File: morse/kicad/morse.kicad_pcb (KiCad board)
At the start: 2 copper layers, 63.5 x 63.5 mm, 14 parts, among them J1 Conn_01x04, Q1 2N2219, Q2 2N2219

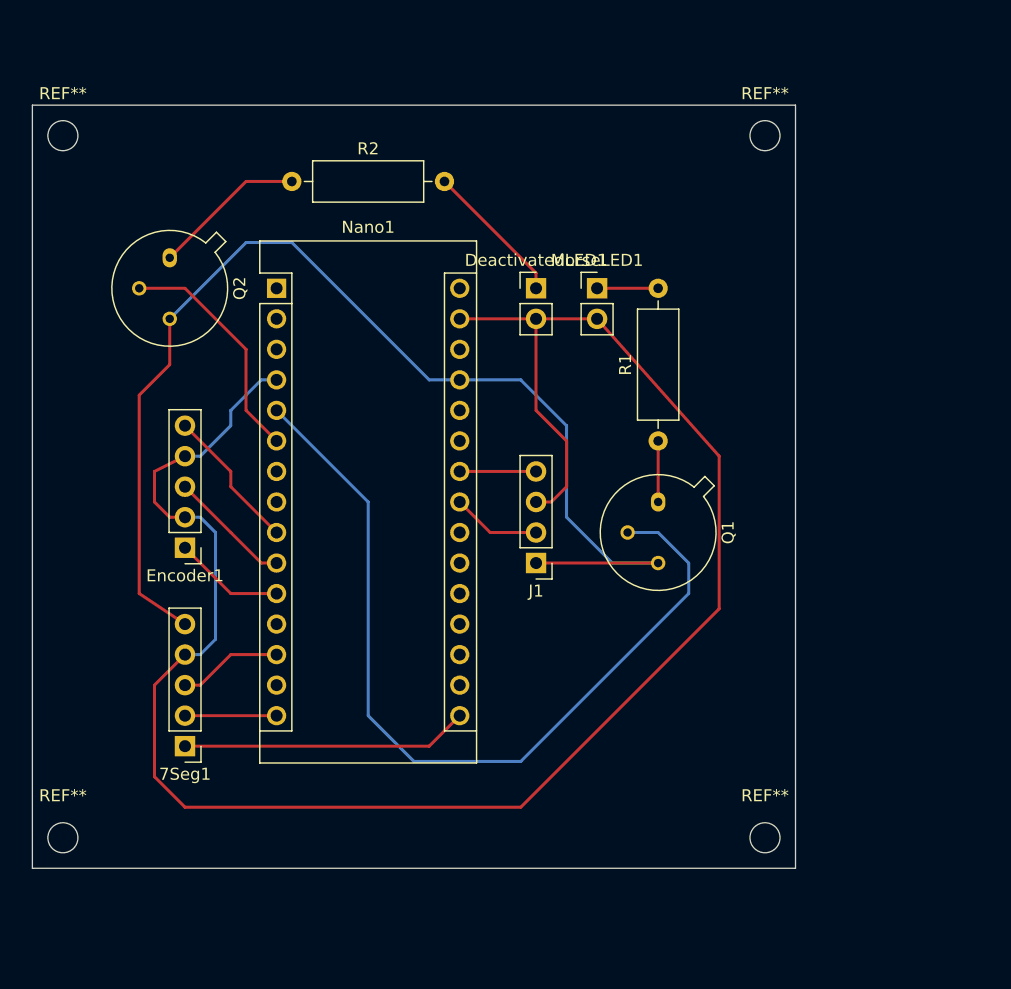
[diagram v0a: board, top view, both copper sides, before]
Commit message: updating morse pcb layout
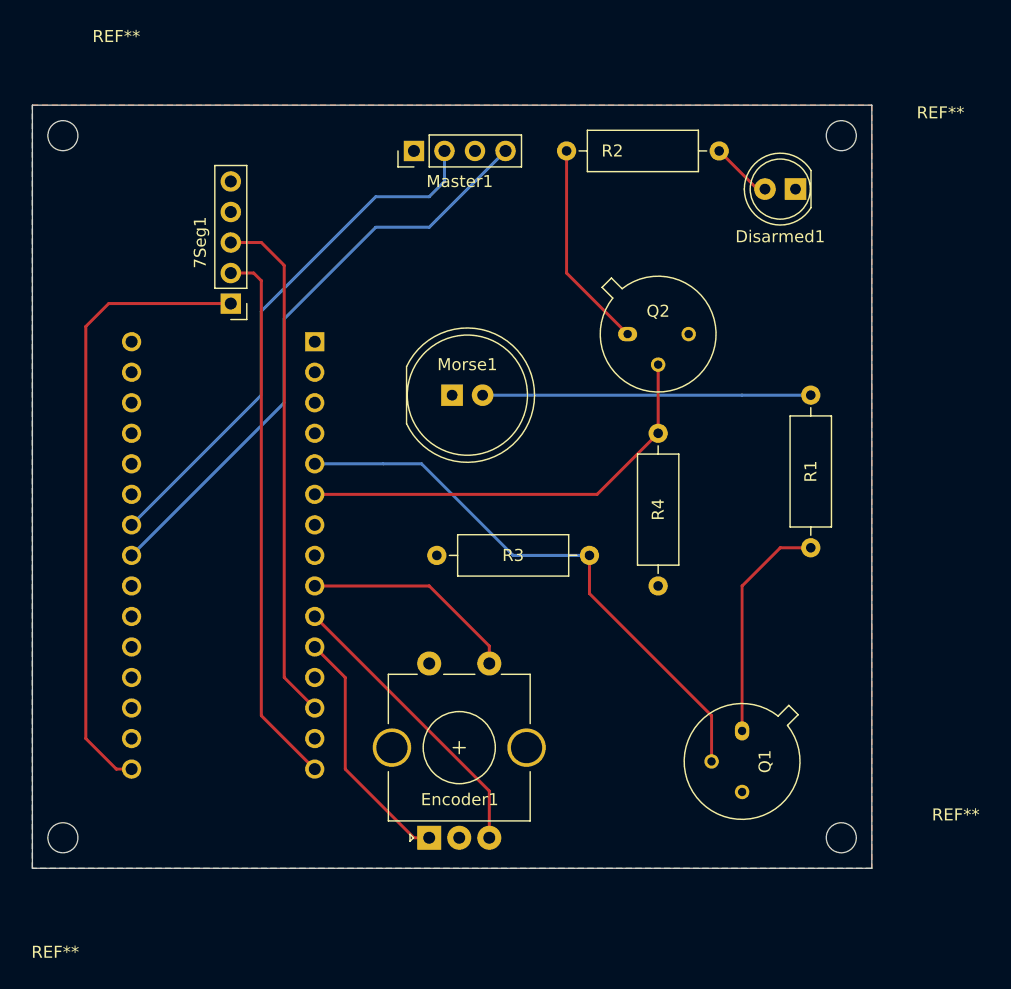
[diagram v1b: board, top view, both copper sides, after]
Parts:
- removed DeactivatedLED1, MorseLED1: Conn_01x02, Connector_PinHeader_2.54mm:PinHeader_1x02_P2.54mm_Vertical
- added Disarmed1: LED, LED_THT:LED_D5.0mm, F.Cu at (196.8, 78.1)
- added Morse1: LED, LED_THT:LED_D10.0mm, F.Cu at (168.3, 95.2)
- added R3: R, Resistor_THT:R_Axial_DIN0309_L9.0mm_D3.2mm_P12.70mm_Horizontal, F.Cu at (179.7, 108.6)
- added R4: R, Resistor_THT:R_Axial_DIN0309_L9.0mm_D3.2mm_P12.70mm_Horizontal, F.Cu at (185.4, 98.4)
- Encoder1: value Conn_01x05 -> Rotary_Encoder_Switch; footprint Connector_PinHeader_2.54mm:PinHeader_1x05_P2.54mm_Vertical -> Rotary_Encoder:RotaryEncoder_Alps_EC11E-Switch_Vertical_H20mm_CircularMountingHoles
- Nano1: moved to B.Cu
- moved Q2 38.6 mm to (182.9, 90.2), turned to 0 degrees
- moved 7Seg1 37.0 mm to (149.9, 87.6)
- moved Master1 35.8 mm to (165.1, 74.9), turned to 90 degrees
- moved Encoder1 31.5 mm to (166.4, 132.1), turned to 90 degrees
- moved R2 23.0 mm to (177.8, 74.9)
- moved Q1 20.3 mm to (192.4, 123.2)
- moved R1 15.5 mm to (198.1, 108.0)
- moved REF** 6.35 mm to (200.7, 132.1)
- moved REF** 6.35 mm to (200.7, 73.7)
- moved Nano1 5.46 mm to (156.8, 90.8), turned to 180 degrees
- renumbered J1 to Master1
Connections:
- Master1 pad 2: Net-(J1-Pad2) -> Net-(Master1-Pad2)
- Master1 pad 4: Net-(J1-Pad4) -> Net-(Master1-Pad4)
- Nano1 pad 10: Net-(Encoder1-Pad3) -> Net-(Encoder1-PadB)
- Nano1 pad 11: Net-(Encoder1-Pad1) -> Net-(Encoder1-PadA)
- Nano1 pad 23: Net-(J1-Pad2) -> Net-(Master1-Pad4)
- Nano1 pad 24: Net-(J1-Pad4) -> Net-(Master1-Pad2)
- Nano1 pad 9: Net-(Encoder1-Pad5) -> Net-(Encoder1-PadS1)
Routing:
- net GND: track 158.1 -> 0.00 mm
- net +5V: track 97.4 -> 0.00 mm
- net Net-(Master1-Pad4): track 0.00 -> 49.1 mm
- net Net-(Master1-Pad2): track 0.00 -> 44.5 mm
- net Net-(7Seg1-Pad2): track 7.62 -> 45.3 mm
- net Net-(7Seg1-Pad3): track 8.67 -> 43.1 mm
- net Net-(7Seg1-Pad1): track 23.9 -> 52.0 mm
- net Net-(Encoder1-PadB): track 0.00 -> 24.4 mm
- net Net-(Nano1-Pad5): track 71.3 -> 47.4 mm
- net Net-(Morse1-Pad2): track 5.08 -> 27.3 mm
- net Net-(Encoder1-PadA): track 0.00 -> 20.6 mm
- net Net-(Encoder1-PadS1): track 0.00 -> 18.1 mm
- net Net-(Nano1-Pad6): track 19.7 -> 36.4 mm
- net Net-(Q1-Pad1): track 5.08 -> 19.1 mm
- net Net-(Encoder1-Pad5): track 12.0 -> 0.00 mm
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- added copper zone on F.Cu, net +5V
- added copper zone on B.Cu, net GND
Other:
- board size 63.5 x 63.5 mm -> 69.8 x 63.5 mm
